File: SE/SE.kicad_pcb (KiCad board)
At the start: 2 copper layers, 43.8 x 49.2 mm, 16 parts, among them J1 RJ45, J2 Conn_01x04_Female, J3 Conn_01x03_Female, Q4 BC548

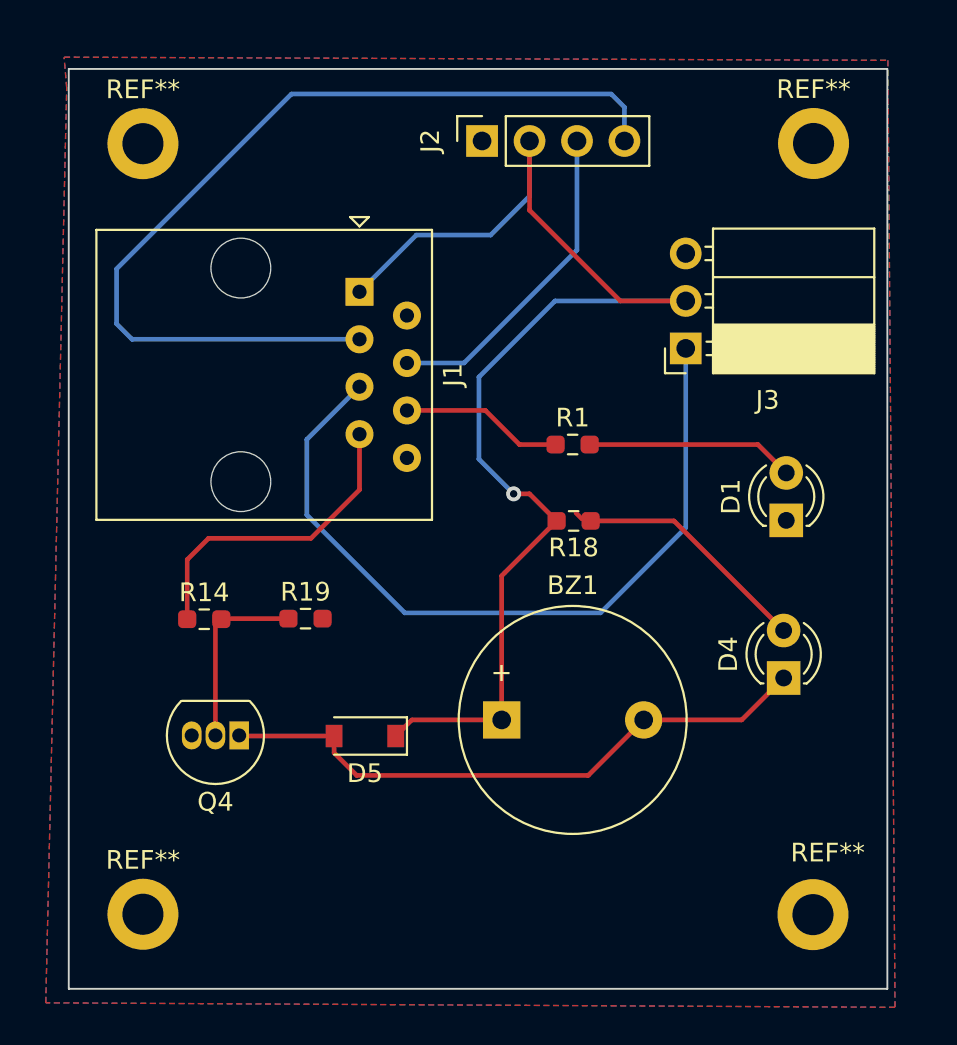
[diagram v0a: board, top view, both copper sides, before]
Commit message: PCB Definitiva
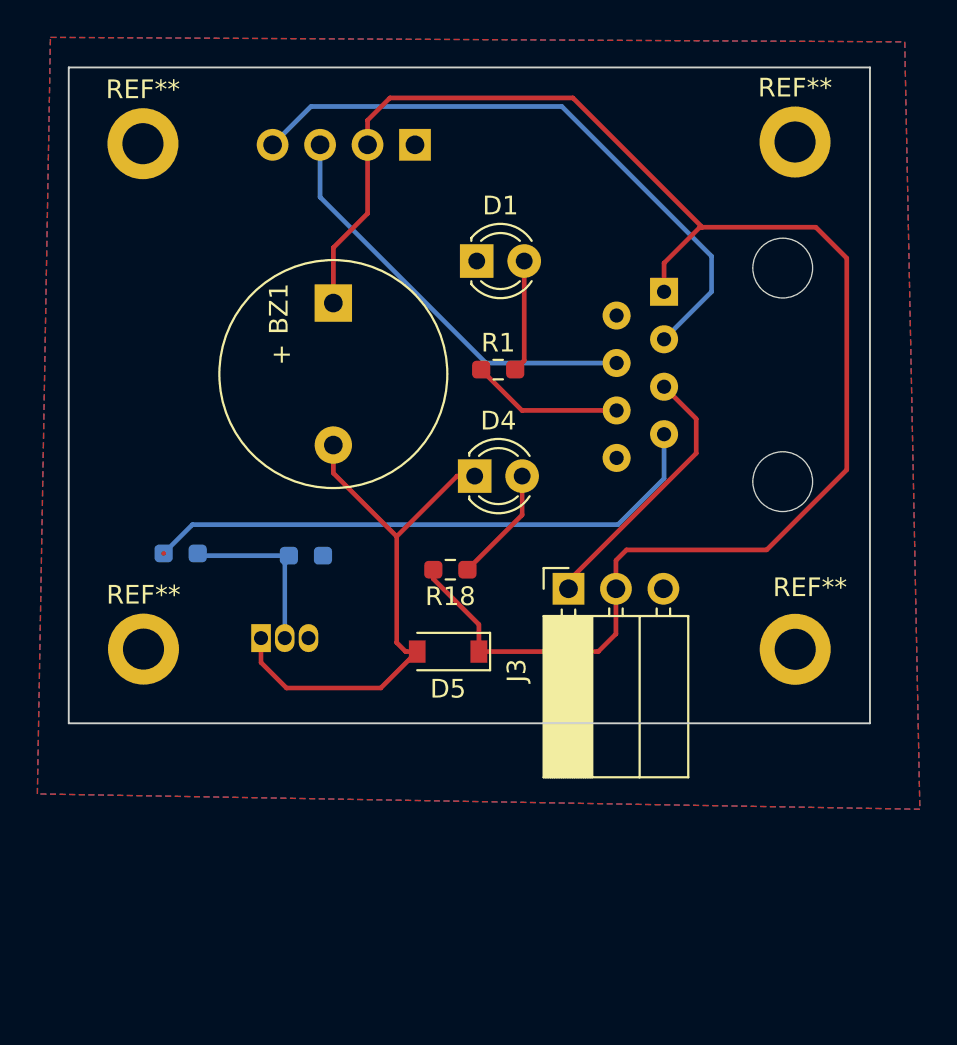
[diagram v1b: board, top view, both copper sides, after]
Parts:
- J1, J2, Q4, R14, R19: moved to B.Cu
- moved BZ1 24.1 mm to (50.9, 47.7), turned to -90 degrees
- moved D1 21.6 mm to (58.6, 45.4), turned to 0 degrees
- moved D4 19.8 mm to (58.5, 57.0), turned to 0 degrees
- moved J1 16.3 mm to (68.6, 47.1)
- moved J3 14.3 mm to (63.5, 63.0), turned to 90 degrees
- moved REF** 14.2 mm to (75.6, 66.2)
- moved REF** 14.2 mm to (40.8, 66.2)
- moved R18 7.10 mm to (57.2, 62.0)
- moved D5 6.34 mm to (57.1, 66.3)
- moved R1 5.65 mm to (59.7, 51.2)
- moved Q4 5.34 mm to (47.0, 65.6), turned to 0 degrees
- moved R14 3.74 mm to (42.8, 61.1)
- moved J2 3.60 mm to (55.3, 39.2)
- moved R19 3.37 mm to (49.5, 61.2)
- moved REF** 0.99 mm to (75.6, 39.1)
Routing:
- net Botones: track 42.0 -> 14.4 mm
- net +3.3V: track 68.8 -> 87.3 mm, vias 1 -> 0
- net SDA: track 49.4 -> 33.2 mm
- net Buzzer: track 16.9 -> 30.8 mm
- net Net-(D4-Pad2): track 13.2 -> 6.22 mm
- net Net-(D1-Pad2): track 11.1 -> 6.01 mm
- net SCL: track 17.4 -> 22.3 mm
- net Net-(BZ1-Pad2): track 32.9 -> 29.8 mm
- net Led_Verde: track 8.71 -> 8.16 mm
- net Net-(Q4-Pad2): track 9.96 -> 9.43 mm
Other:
- board size 43.8 x 49.2 mm -> 42.9 x 35.1 mm
